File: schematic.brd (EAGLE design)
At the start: 60.9 x 63.2 mm, 40 parts, among them CN1 1X4-BIG, CN2 1X4-BIG, IC3 78TO220, IC4 78TO220

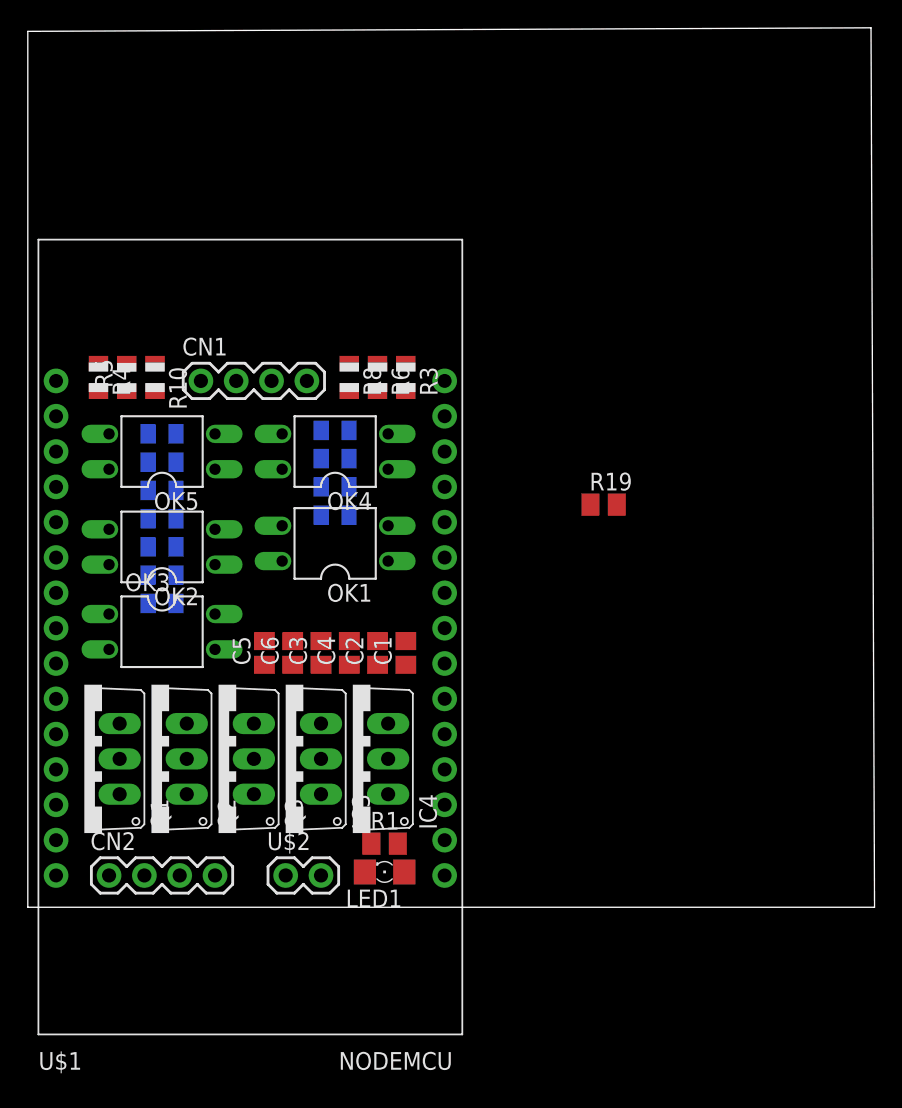
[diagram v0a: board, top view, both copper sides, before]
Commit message: Initial board layout
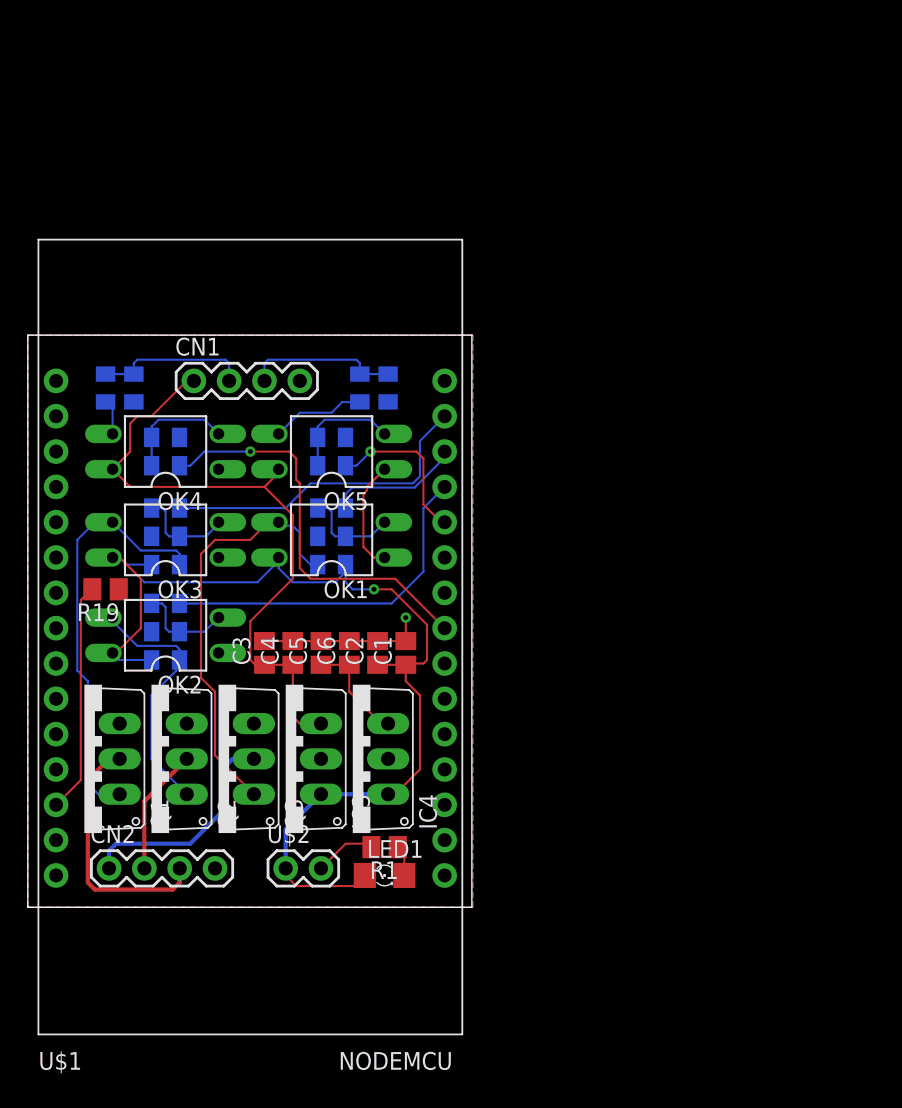
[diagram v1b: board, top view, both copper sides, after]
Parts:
- moved R19 36.3 mm to (4.83, 21.8), turned to 180 degrees
- moved R3 25.2 mm to (9.14, 18.8), flipped to the bottom, turned to 180 degrees
- moved R8 24.2 mm to (9.14, 16.8), flipped to the bottom, turned to 180 degrees
- moved R6 22.3 mm to (9.14, 20.8), flipped to the bottom, turned to 180 degrees
- moved R18 18.8 mm to (25.1, 36.3), turned to 90 degrees
- moved R13 17.3 mm to (4.83, 36.3), turned to 270 degrees
- moved R17 17.1 mm to (6.86, 36.3), turned to 90 degrees
- moved R14 15.2 mm to (23.1, 36.3), turned to 270 degrees
- moved R10 13.5 mm to (9.14, 23.6), flipped to the bottom, turned to 180 degrees
- moved R2 13.1 mm to (21.1, 25.7)
- moved R7 13.1 mm to (21.1, 27.7), turned to 180 degrees
- moved R4 12.4 mm to (9.14, 25.7), flipped to the bottom, turned to 180 degrees
- moved R15 12.3 mm to (21.1, 30.7)
- moved R16 12.3 mm to (9.14, 30.7), turned to 180 degrees
- moved R9 12.3 mm to (21.1, 23.6), turned to 0 degrees
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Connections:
- net CTRL_A_3V3: now also U$1.P$23; no longer U$1.P$26
- net CTRL_B_3V3: now also U$1.P$26; no longer U$1.P$23
- net CTRL_G: now also U$1.P$27; no longer U$1.P$28
- net CTRL_R: now also U$1.P$28; no longer U$1.P$27
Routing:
- net +12V: track 0.00 -> 77.9 mm, vias 0 -> 1
- net +5V: track 0.00 -> 46.5 mm
- net N$7: track 0.00 -> 30.4 mm
- net N$5: track 0.00 -> 30.1 mm
- net CTRL_A_3V3: track 0.00 -> 29.2 mm, vias 0 -> 1
- net CTRL_G: track 0.00 -> 25.2 mm
- net CTRL_B: track 0.00 -> 23.3 mm
- net POW_B: track 0.00 -> 18.3 mm
- net N$6: track 0.00 -> 18.2 mm
- net N$8: track 0.00 -> 16.6 mm
- net POW_R: track 0.00 -> 16.4 mm
- net GND: track 0.00 -> 16.3 mm, vias 0 -> 1
- net +3V3: track 0.00 -> 15.8 mm
- net CTRL_B_3V3: track 0.00 -> 11.6 mm, vias 0 -> 1
- net CTRL_B_5V: track 0.00 -> 11.1 mm
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- added copper zone on layer 1, net +3V3
- added copper zone on layer 16, net GND
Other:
- board size 60.9 x 63.2 mm -> 31.9 x 41.1 mm
